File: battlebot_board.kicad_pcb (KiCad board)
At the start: 4 copper layers, 60 x 45 mm, 44 parts, among them J1 Conn_01x02_Pin, J2 Conn_01x04_Pin, J3 JST_SMD_1.0mm_Vertical, J4 Conn_01x02, J5 JST_02, J6 JST_02, Q1 AO3400A, Q2 AO3400A, SW1 Switch_Tactile_CnK, U1 AP63203WU, U2 LPC824M201JHI33, U3 TMP102, U4 LSM6DSOX, U5 W25Q128JVP

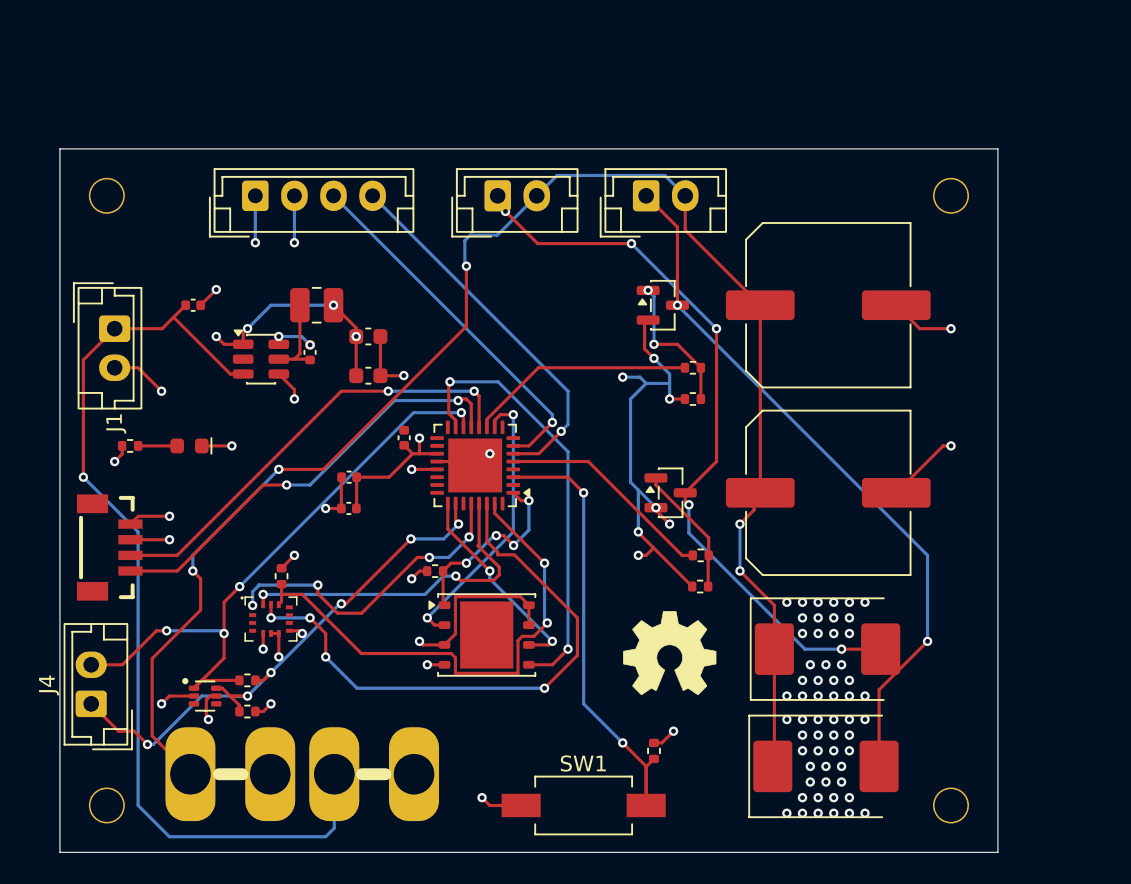
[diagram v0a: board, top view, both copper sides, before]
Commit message: redesign
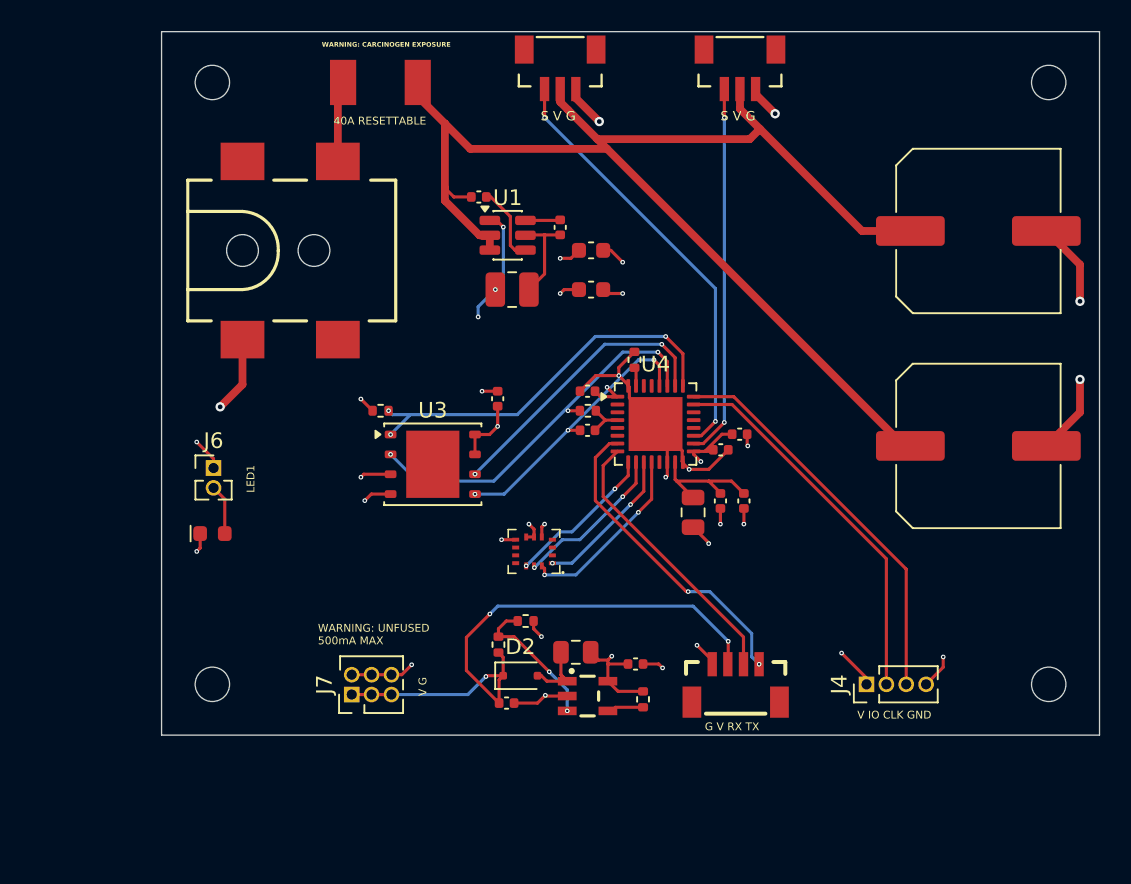
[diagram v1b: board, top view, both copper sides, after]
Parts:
- removed D3: Green, PCM_SparkFun-LED:LED_0603_1608Metric_Green
- removed D4, D5: B340, Diode_SMD:D_SMC
- removed F4: Blade Fuse, PCM_SparkFun-Fuse:Fuseholder_Automotive
- removed G***: LOGO, LOGO
- removed H1, H2, H3, H4: ~, PCM_fab:MountingHole_M2
- removed Q1, Q2: AO3400A, Package_TO_SOT_SMD:SOT-23
- removed R10, R7, R9: 10k, PCM_SparkFun-Resistor:R_0402_1005Metric
- removed R8: 100, PCM_SparkFun-Resistor:R_0402_1005Metric
- removed Ref**: Val**, PCM_SparkFun-Aesthetic:OSHW_Logo_6mm
- removed SW1: Switch_Tactile_CnK, PCM_fab:Button_CnK_PTS636.0_6x3.5mm
- added C11: 0.1uF, PCM_SparkFun-Capacitor:C_0402_1005Metric, F.Cu at (146.5, 97.0)
- added C13: 470uF, PCM_SparkFun-Capacitor:Electrolytic_10.3x10.3mm, F.Cu at (177.2, 100.0)
- added C14: 0.1uF, PCM_SparkFun-Capacitor:C_0402_1005Metric, F.Cu at (155.3, 114.0)
- added C15: 1.0uF, PCM_SparkFun-Capacitor:C_0402_1005Metric, F.Cu at (147.1, 116.5)
- added C6: 0.1uF, PCM_SparkFun-Capacitor:C_0402_1005Metric, F.Cu at (162.0, 99.2)
- added C9: 10nF, PCM_SparkFun-Capacitor:C_0402_1005Metric, F.Cu at (162.2, 103.5)
- added D1: Green, PCM_SparkFun-LED:LED_0603_1608Metric_Green, F.Cu at (128.3, 105.6)
- added D2: PMEG4005EJ, Diode_SMD:D_SOD-323F, F.Cu at (148.0, 114.7)
- added F1: 16V/2.5A/5.0A, PCM_SparkFun-Fuse:1812, F.Cu at (139.0, 76.8)
- added J7: Conn_02x03, Connector_PinHeader_1.27mm:PinHeader_2x03_P1.27mm_Vertical, F.Cu at (137.2, 115.9)
- added L2: 600 Ohm, PCM_SparkFun-Capacitor:C_0805_2012Metric, F.Cu at (159.0, 104.2)
- added L3: 10uH, PCM_SparkFun-Capacitor:C_0805_2012Metric, F.Cu at (151.5, 113.2)
- added REF**: MountingHole_2.2mm_M2_DIN965, MountingHole:MountingHole_2.2mm_M2_DIN965, F.Cu at (128.2, 115.2)
- added REF**: MountingHole_2.2mm_M2_DIN965, MountingHole:MountingHole_2.2mm_M2_DIN965, F.Cu at (181.8, 76.8)
- added REF**: MountingHole_2.2mm_M2_DIN965, MountingHole:MountingHole_2.2mm_M2_DIN965, F.Cu at (181.8, 115.2)
- added REF**: MountingHole_2.2mm_M2_DIN965, MountingHole:MountingHole_2.2mm_M2_DIN965, F.Cu at (128.2, 76.8)
- C1, C2: value 10uF -> 0.1uF
- C10: value 470uF -> 0.1uF; footprint PCM_SparkFun-Capacitor:Electrolytic_10.3x10.3mm -> PCM_SparkFun-Capacitor:C_0402_1005Metric
- C3: value 0.1uF -> 22uF; footprint PCM_SparkFun-Capacitor:C_0402_1005Metric -> PCM_SparkFun-Capacitor:C_0603_1608Metric
- C5: value 22uF -> 0.1uF; footprint PCM_SparkFun-Capacitor:C_0603_1608Metric -> PCM_SparkFun-Capacitor:C_0402_1005Metric
- C7: value 0.1uF -> 10uF
- C8: value 0.1uF -> 1.0uF
- J1: value Conn_01x02_Pin -> Conn_01x03_Socket; footprint Connector_JST:JST_EH_B2B-EH-A_1x02_P2.50mm_Vertical -> PCM_SparkFun-Connector:JST_1x03_P1.0mm_Vertical_SMD
- J2: value Conn_01x04_Pin -> Barrel_Jack_SMD; footprint Connector_JST:JST_EH_B4B-EH-A_1x04_P2.50mm_Vertical -> PCM_SparkFun-Connector:Barrel_Jack_SMD
- J3: value JST_SMD_1.0mm_Vertical -> Conn_01x03_Socket; footprint PCM_SparkFun-Connector:JST_1x04_P1.0mm_Vertical_SMD -> PCM_SparkFun-Connector:JST_1x03_P1.0mm_Vertical_SMD
- J4: value Conn_01x02 -> Conn_01x04_Pin; footprint Connector_JST:JST_EH_B2B-EH-A_1x02_P2.50mm_Vertical -> Connector_PinHeader_1.27mm:PinHeader_1x04_P1.27mm_Vertical
- J5: value JST_02 -> Conn_01x04_Socket; footprint Connector_JST:JST_EH_B2B-EH-A_1x02_P2.50mm_Vertical -> PCM_SparkFun-Connector:JST_1x04_P1.0mm_Vertical_SMD
- J6: value JST_02 -> Conn_01x02_Pin; footprint Connector_JST:JST_EH_B2B-EH-A_1x02_P2.50mm_Vertical -> Connector_PinHeader_1.27mm:PinHeader_1x02_P1.27mm_Vertical
- R4, R5: value 4.7k -> 100k
- R6: value 100 -> 33k
- U2: value LPC824M201JHI33 -> LSM6DSOX; footprint Package_DFN_QFN:QFN-32-1EP_5x5mm_P0.5mm_EP3.45x3.45mm -> PCM_SparkFun-Sensor:ST_LGA-14L_2.5x3.0mm_P0.5mm_4x3
- U3: value TMP102 -> W25Q128JVP; footprint PCM_SparkFun-Semiconductor-Standard:SOT-563 -> Package_SON:WSON-8-1EP_6x5mm_P1.27mm_EP3.4x4.3mm
- U4: value LSM6DSOX -> STM32G4A1KEUx; footprint PCM_SparkFun-Sensor:ST_LGA-14L_2.5x3.0mm_P0.5mm_4x3 -> Package_DFN_QFN:QFN-32-1EP_5x5mm_P0.5mm_EP3.45x3.45mm
- U5: value W25Q128JVP -> AP3012; footprint Package_SON:WSON-8-1EP_6x5mm_P1.27mm_EP3.4x4.3mm -> PCM_SparkFun-Semiconductor-Standard:SOT23-5
- moved J4 49.6 mm to (170.1, 115.2)
- moved J1 44.2 mm to (162.0, 73.7), turned to 0 degrees
- moved J3 43.7 mm to (150.5, 73.7), turned to 0 degrees
- moved J5 32.0 mm to (161.7, 115.5), turned to 180 degrees
- moved U4 27.6 mm to (156.6, 98.6)
- moved R4 25.3 mm to (155.8, 116.2), turned to 90 degrees
- moved J6 25.2 mm to (128.3, 101.4)
- moved C2 24.0 mm to (150.5, 86.0), turned to -90 degrees
- moved C8 23.8 mm to (160.8, 103.5), turned to -90 degrees
- moved R1 22.2 mm to (152.3, 97.8), turned to 180 degrees
- moved U3 20.8 mm to (142.3, 101.2)
- moved C7 20.3 mm to (160.8, 100.2), turned to 0 degrees
- moved C1 19.8 mm to (145.3, 84.1), turned to 0 degrees
- moved R6 19.4 mm to (148.3, 111.2), turned to 180 degrees
- moved C12 19.3 mm to (177.2, 86.2)
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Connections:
- C1 pad 1: 3.3V -> VIN
- C10 pad 1: Net-(D4-K) -> /NRST
- C12 pad 1: Net-(D4-K) -> VIN
- C2 pad 1: 12V -> Net-(U1-BST)
- C2 pad 2: GND -> Net-(U1-SW)
- C3 pad 1: Net-(U1-BST) -> 3.3V
- C3 pad 2: Net-(U1-SW) -> GND
- C7 pad 1: GND -> 3.3V
- C7 pad 2: 3.3V -> GND
- C8 pad 1: GND -> Net-(U4-VDDA)
- C8 pad 2: 3.3V -> GND
- J1 pad 1: 12V -> /CH1
- J1 pad 2: GND -> VIN
- J3 pad 1: /TXD -> /CH2
- J3 pad 2: /RXD -> VIN
- J3 pad 3: 3.3V -> GND
- J4 pad 1: /SDA1 -> 3.3V
- J4 pad 2: /SCL1 -> /SWDIO
- J5 pad 1: Net-(D5-A) -> /TX2
- J5 pad 2: Net-(D4-K) -> /RX2
- J6 pad 1: Net-(D4-A) -> 3.3V
- J6 pad 2: Net-(D4-K) -> Net-(D1-A)
- R2 pad 1: /CS1 -> GND
- R2 pad 2: 3.3V -> /BOOT0
- R4 pad 1: /SCL1 -> Net-(U5-~{SHDN})
- R5 pad 1: /SDA1 -> Net-(U5-FB)
- R5 pad 2: 3.3V -> 5V
- R6 pad 1: /MOTOR1 -> GND
- R6 pad 2: Net-(Q1-G) -> Net-(U5-FB)
- U1 pad 2: unconnected-(U1-EN-Pad2) -> VIN
- U1 pad 3: 12V -> VIN
- U2 pad 1: /CS1 -> /MISO
- U2 pad 10: /MISO1 -> unconnected-(U2-OCS_Aux-Pad10)
- U2 pad 11: /MOTOR1 -> unconnected-(U2-SDO_Aux-Pad11)
- U2 pad 12: /RXD -> /CS
- U2 pad 13: /TXD -> /SCK
- U2 pad 14: /SCL1 -> /MOSI
- U2 pad 3: /NRST -> unconnected-(U2-SCx-Pad3)
- U2 pad 5: /MOTOR2 -> 3.3V
- U2 pad 6: /SWCLK -> GND
- U2 pad 7: /SWDIO -> GND
- U2 pad 8: unconnected-(U2-PIO0_11-Pad8) -> 3.3V
- U3 pad 1: /SCL1 -> /CS2
- U3 pad 2: GND -> /MISO2
- U3 pad 3: unconnected-(U3-ALERT-Pad3) -> 3.3V
- U3 pad 4: unconnected-(U3-ADD0-Pad4) -> GND
- U3 pad 5: 3.3V -> /MOSI2
- U3 pad 6: /SDA1 -> /SCK2
- U4 pad 1: /MISO2 -> 3.3V
- U4 pad 10: unconnected-(U4-OCS_Aux-Pad10) -> /SCK
- U4 pad 11: unconnected-(U4-SDO_Aux-Pad11) -> /MISO
- U4 pad 12: /CS2 -> /MOSI
- U4 pad 13: /SCK2 -> unconnected-(U4-PB0-Pad13)
- U4 pad 14: /MOSI2 -> GND
- U4 pad 4: unconnected-(U4-INT1-Pad4) -> /NRST
- U4 pad 5: 3.3V -> unconnected-(U4-PA0-Pad5)
- U4 pad 6: GND -> unconnected-(U4-PA1-Pad6)
- U4 pad 7: GND -> /TX2
- U4 pad 8: 3.3V -> /RX2
- U4 pad 9: unconnected-(U4-INT2-Pad9) -> /CS
- U5 pad 1: /CS1 -> Net-(D2-A)
- U5 pad 2: /MISO1 -> GND
- U5 pad 3: 3.3V -> Net-(U5-FB)
- U5 pad 4: GND -> Net-(U5-~{SHDN})
- U5 pad 5: /MOSI1 -> 3.3V
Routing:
- net Net-(D4-K): track 106.9 -> 0.00 mm, vias 5 -> 0
- net VIN: track 0.00 -> 84.4 mm
- net 12V: track 66.1 -> 0.00 mm, vias 1 -> 0
- net Net-(D4-A): track 47.2 -> 0.00 mm, vias 5 -> 0
- net Net-(D5-A): track 45.2 -> 0.00 mm, vias 2 -> 0
- net /SCL1: track 40.1 -> 0.00 mm, vias 4 -> 0
- net 5V: track 0.00 -> 38.7 mm, vias 0 -> 3
- net /SDA1: track 35.4 -> 0.00 mm, vias 5 -> 0
- net /RXD: track 28.8 -> 0.00 mm, vias 2 -> 0
- net /MOSI1: track 28.1 -> 0.00 mm, vias 2 -> 0
- net /TXD: track 28.0 -> 0.00 mm, vias 2 -> 0
- net /CH2: track 0.00 -> 27.6 mm, vias 0 -> 2
- net /NRST: track 29.8 -> 2.55 mm, vias 2 -> 0
- net /CH1: track 0.00 -> 23.9 mm, vias 0 -> 2
- net /TX2: track 0.00 -> 20.2 mm, vias 0 -> 2
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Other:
- board text added: "40A RESETTABLE"
- board text added: "G V RX TX"
- board text added: "LED1"
- board text added: "S V G"
- board text added: "V G"
- board text added: "V IO CLK GND"
- board text added: "WARNING: CARCINOGEN EXPOSURE"
- board text added: "WARNING: UNFUSED 500mA MAX"
- board text removed: "Antweight Controller V1"
- board text removed: "Designed by Benjamin Liu"
- board text removed: "GND 12V"
- board text removed: "SDA SCL"
- board text removed: "T R V G"
- board text removed: "V G SWDIO SWCLK"
